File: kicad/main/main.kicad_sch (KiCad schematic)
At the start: 52 parts, among them J1 to cam, J10 I2C_1, J11 drib-kick, J12 drib-kick, J14 5V OUT, J15 LINE, J3 USB_C_Receptacle_USB2.0, J4 Power IN, J5 MD1, J6 MD2, J7 Serial0/XBee, J8 Serial1/IMU, J9 AUX1, Q1 AO3400A, Q2 AO3401A, SW1 BTN_UP, SW2 BTN_UP, SW3 Reset, U2 RP2040_Stamp, U3 74HC32, U4 74HC04, U5 OKL-T_3-W12N-C

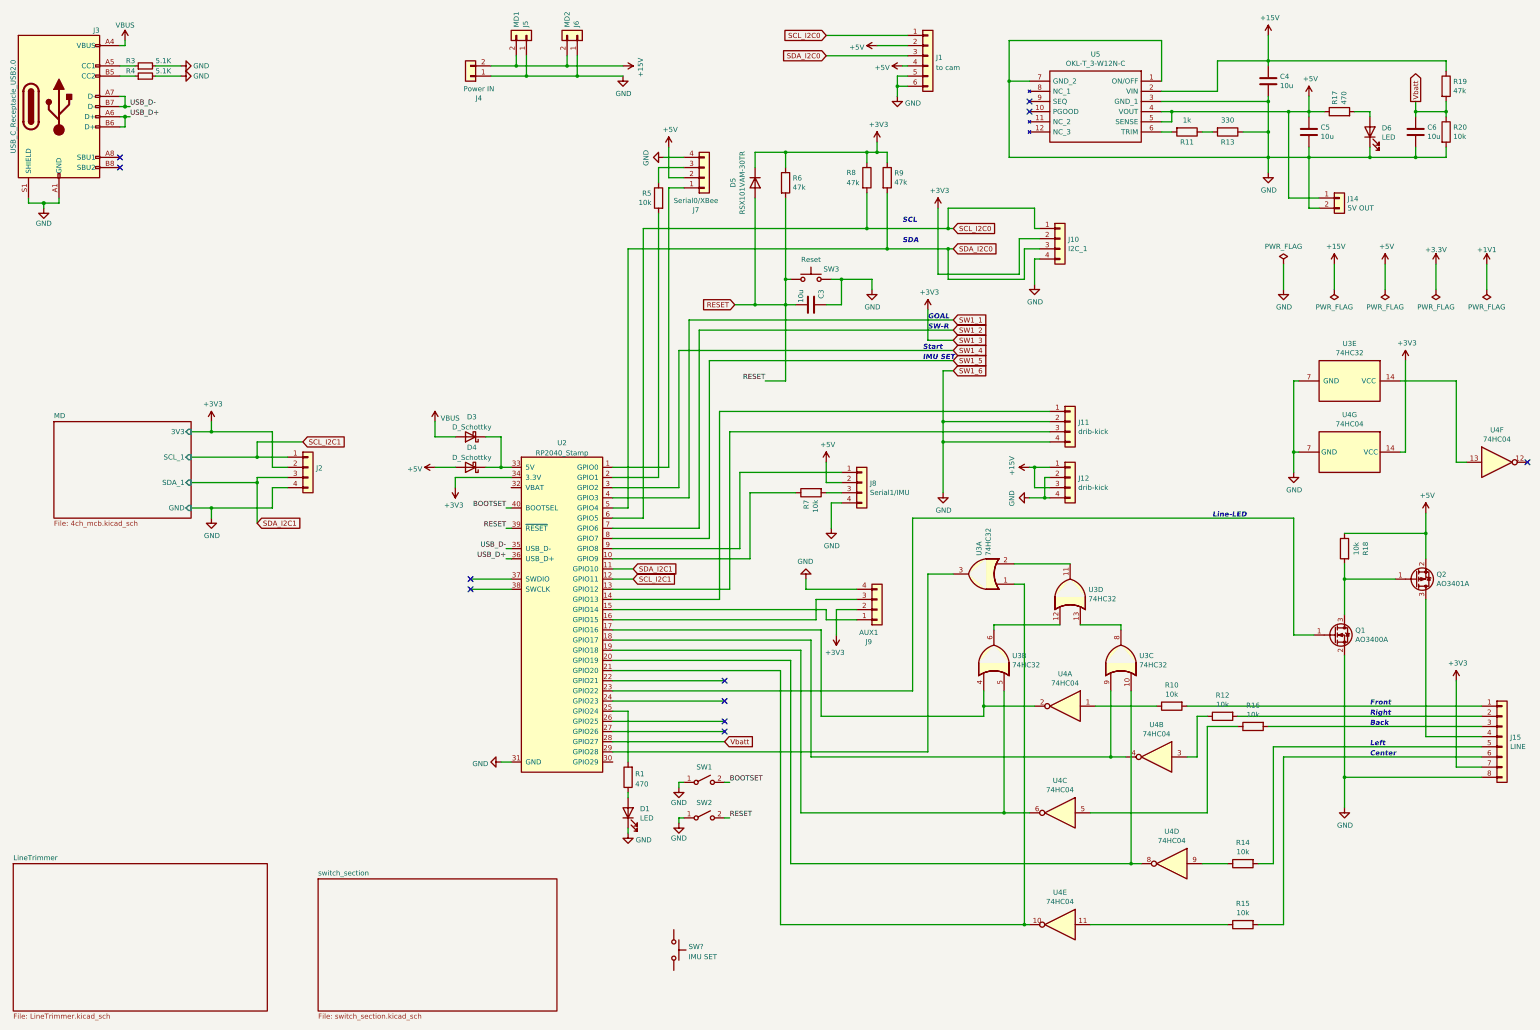
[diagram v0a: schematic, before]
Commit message: main bus
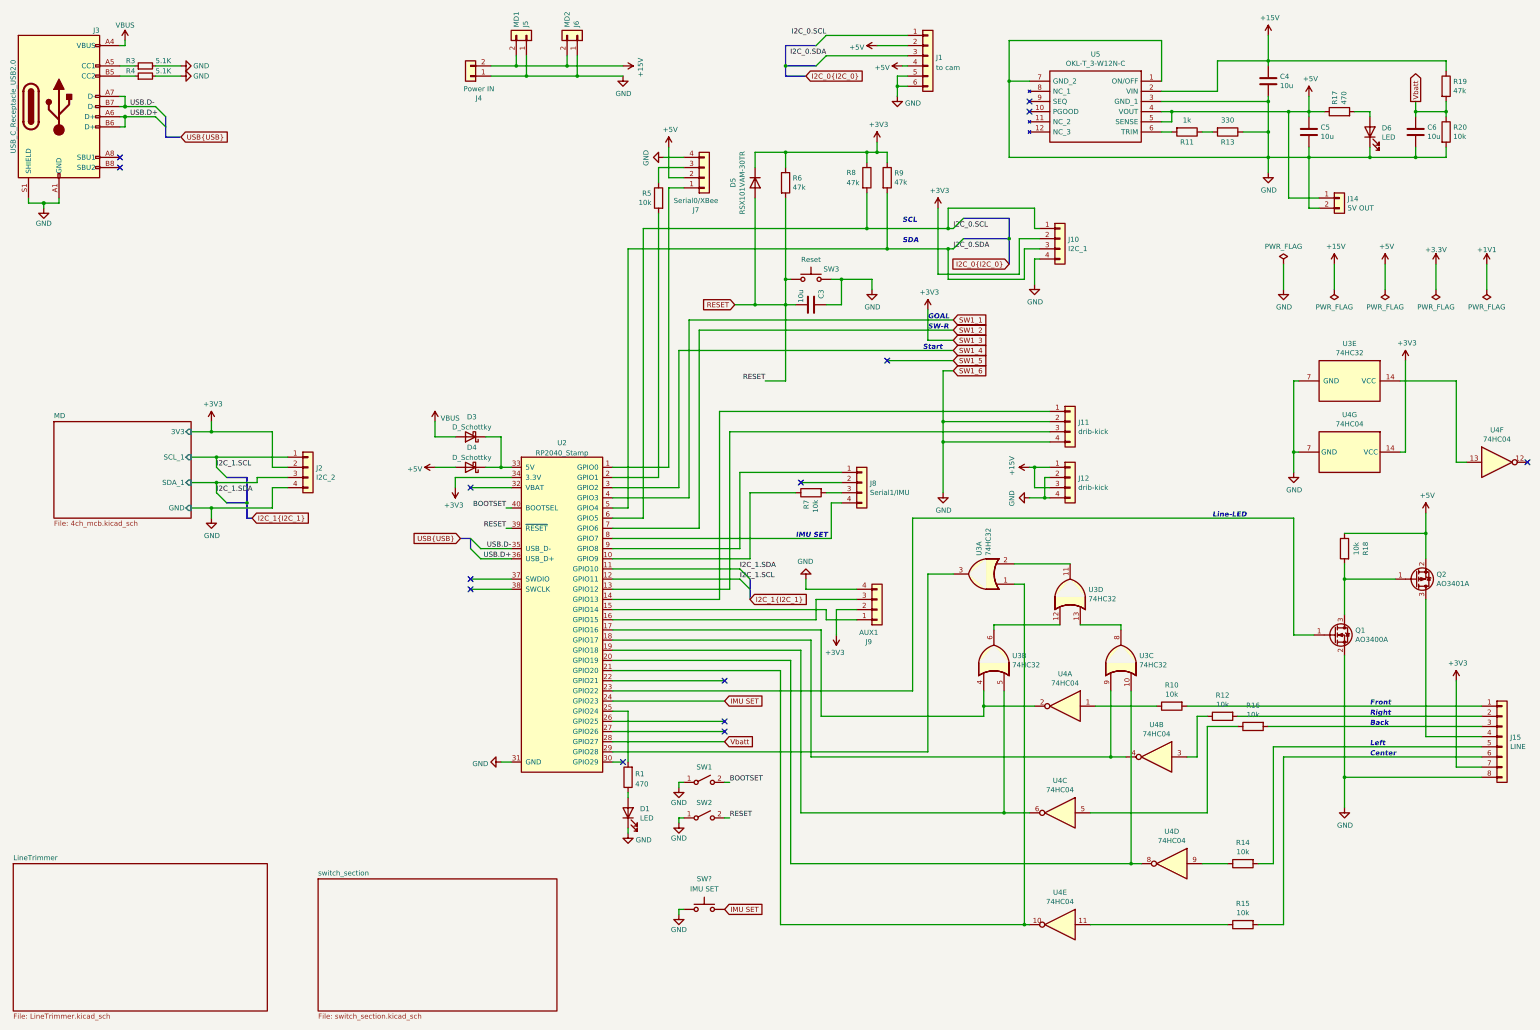
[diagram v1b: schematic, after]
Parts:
- J2: value (none) -> I2C_2; footprint (none) -> 0.main.robot:JSTB4B-ZR
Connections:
- net +5V: no longer J8.2 (Pin_2)
- net GND: now also SW?.1; no longer J8.4 (Pin_4)
- net SW1_5: no longer U2.8 (GPIO7)
- net IMU SET: now reaches SW?.2
- net IMU SET: now also U2.24 (GPIO23)
- net SCL_I2C0 renamed I2C_0.SCL
- net SCL_I2C1 renamed I2C_1.SCL
- net SDA_I2C0 renamed I2C_0.SDA
- net SDA_I2C1 renamed I2C_1.SDA
- net USB_D+ renamed USB.D+
- net USB_D- renamed USB.D-
- new net: J8.4 (Pin_4), U2.8 (GPIO7)
- no-connect marks 11 -> 14
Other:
- moved on the sheet: SW?
